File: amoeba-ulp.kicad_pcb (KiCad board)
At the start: 2 copper layers, 18.2 x 16.8 mm, 6 parts

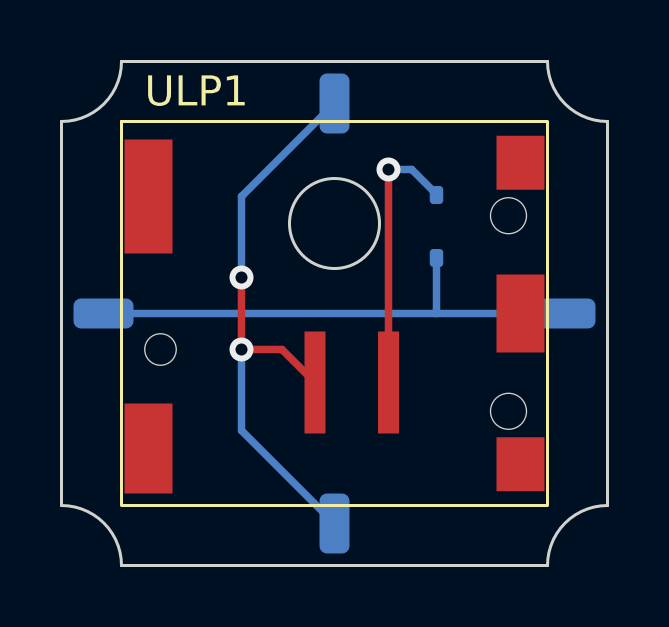
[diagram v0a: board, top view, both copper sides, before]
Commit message: kailh switch version
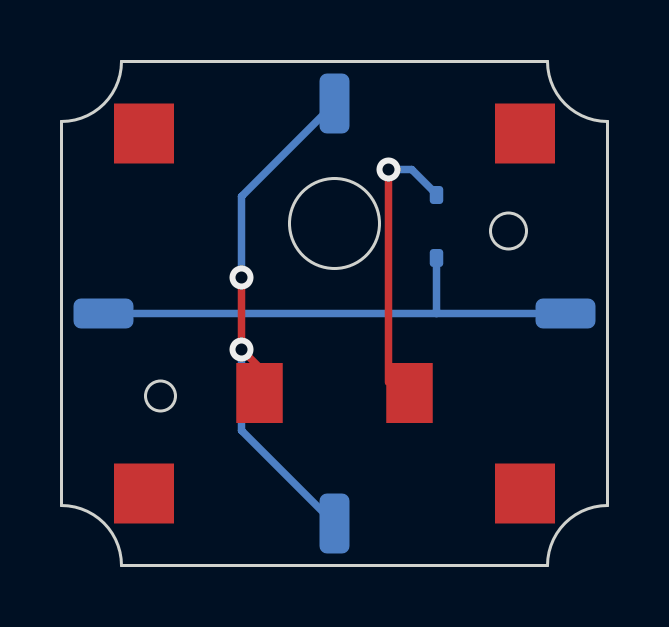
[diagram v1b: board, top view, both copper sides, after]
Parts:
- ULP1: footprint Cherry_MX_ULP:Cherry_ULP_SMD -> Kailh_ULP:CPG1316S01D02_mikeholscher
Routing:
- net Column: track 19.5 -> 18.3 mm
